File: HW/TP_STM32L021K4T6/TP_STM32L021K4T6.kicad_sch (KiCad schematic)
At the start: 16 parts, among them U1 STM32L021K4Tx, U2 BU33SD5WG-TR

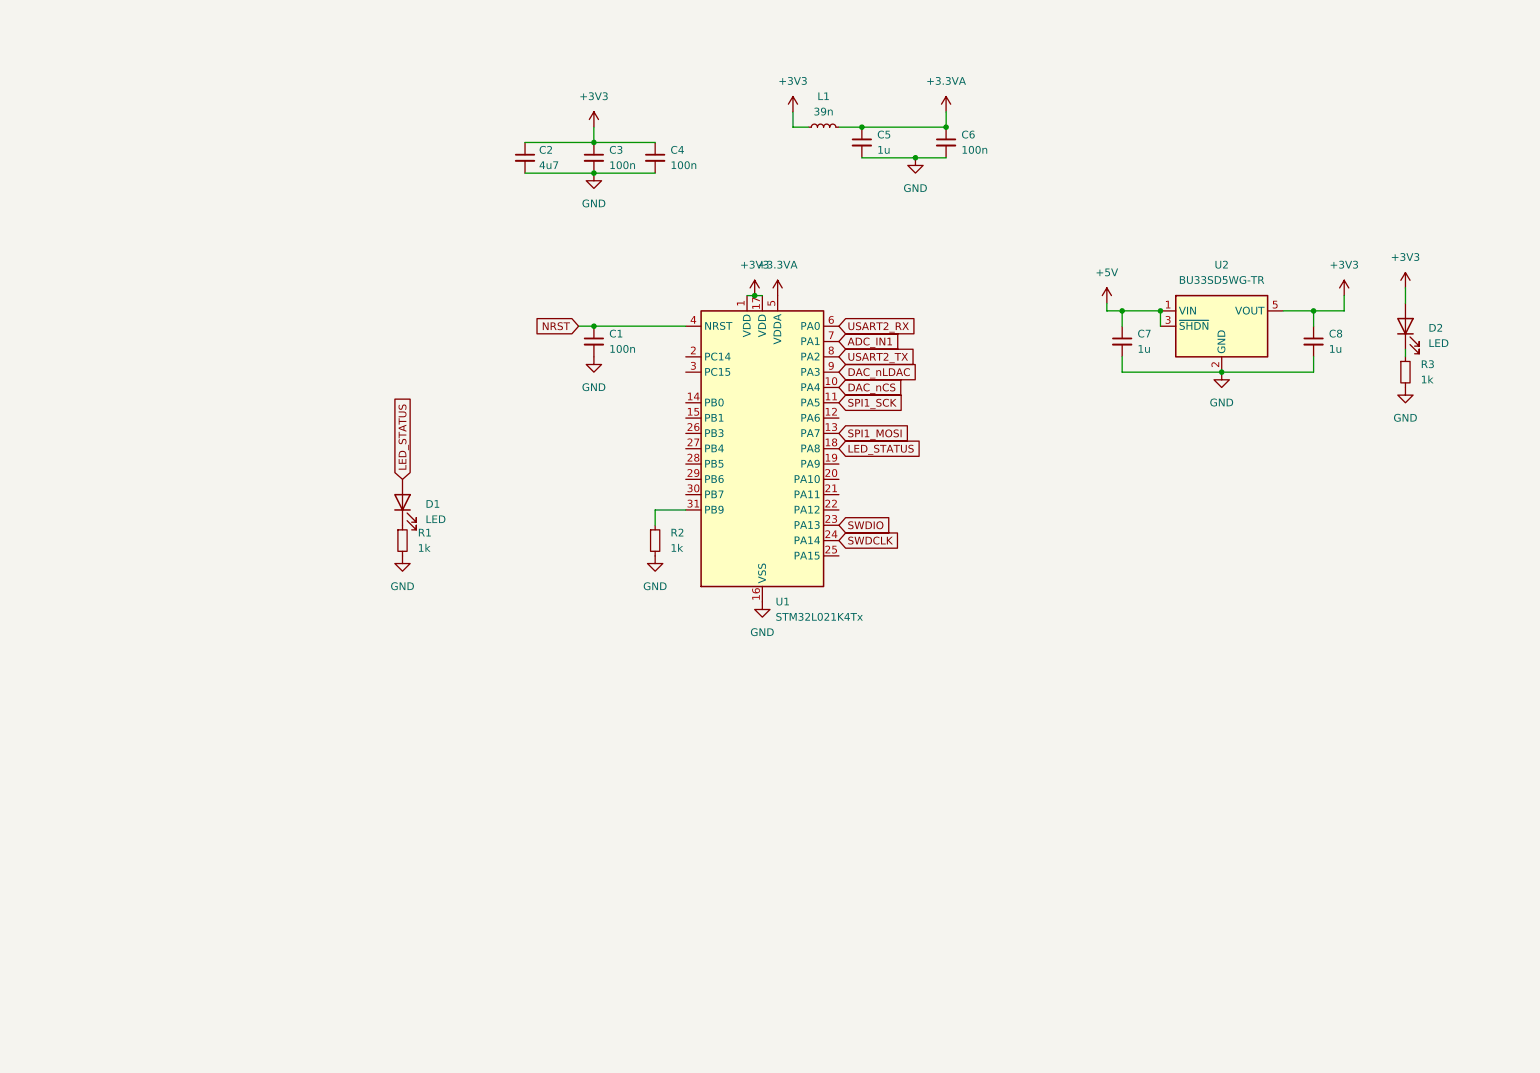
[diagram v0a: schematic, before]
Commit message: Save PCB
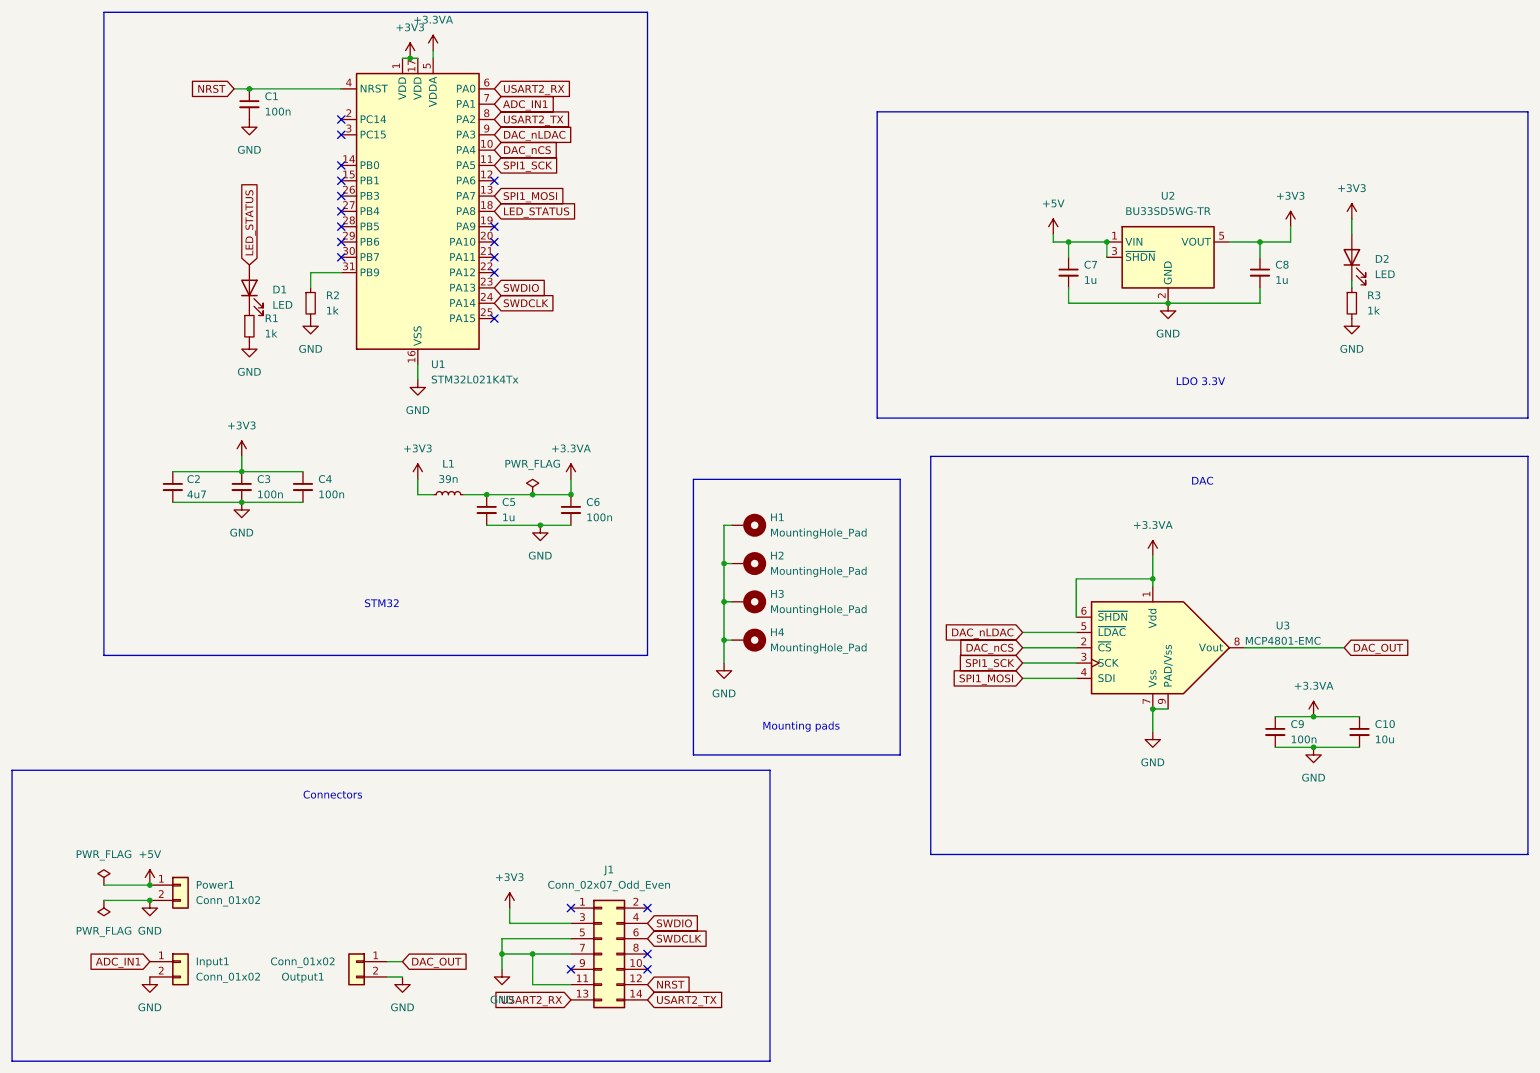
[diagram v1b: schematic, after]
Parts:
- added C10: 10u, Capacitor_SMD:C_0805_2012Metric, symbol Device:C_Small
- added C9: 100n, Capacitor_SMD:C_0805_2012Metric_Pad1.18x1.45mm_HandSolder, symbol Device:C_Small
- added H1, H2, H3, H4: MountingHole_Pad, MountingHole:MountingHole_3.2mm_M3_Pad, symbol Mechanical:MountingHole_Pad
- added Input1, Output1, Power1: Conn_01x02, Connector_JST:JST_XH_B2B-XH-AM_1x02_P2.50mm_Vertical, symbol Connector_Generic:Conn_01x02
- added J1: Conn_02x07_Odd_Even, Connector_PinHeader_1.27mm:PinHeader_2x07_P1.27mm_Vertical_SMD, symbol Connector_Generic:Conn_02x07_Odd_Even
- added U3: MCP4801-EMC, Package_DFN_QFN:DFN-8-1EP_3x2mm_P0.5mm_EP1.75x1.45mm, symbol Analog_DAC:MCP4801-EMC
- C1, C2, C3, C4, C6: footprint (none) -> Capacitor_SMD:C_0805_2012Metric_Pad1.18x1.45mm_HandSolder
- C5, C7, C8: footprint (none) -> Capacitor_SMD:C_0805_2012Metric
- D1, D2: footprint (none) -> LED_SMD:LED_0201_0603Metric_Pad0.64x0.40mm_HandSolder
- L1: footprint (none) -> Inductor_SMD:L_0805_2012Metric_Pad1.05x1.20mm_HandSolder
- R1, R2, R3: footprint (none) -> Resistor_SMD:R_0805_2012Metric_Pad1.20x1.40mm_HandSolder
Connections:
- net +3.3VA: now also C10.1, C9.1, U3.1 (Vdd), U3.6 (~{SHDN})
- net +3V3: now also J1.3 (Pin_3)
- net +5V: now also Power1.1 (Pin_1)
- net ADC_IN1: now also Input1.1 (Pin_1)
- net DAC_nCS: now also U3.2 (~{CS})
- net DAC_nLDAC: now also U3.5 (~{LDAC})
- net GND: now also C10.2, C9.2, H1.1, H2.1, H3.1, H4.1, Input1.2 (Pin_2), J1.11 (Pin_11), J1.5 (Pin_5), J1.7 (Pin_7), Output1.2 (Pin_2), Power1.2 (Pin_2), U3.7 (Vss), U3.9 (PAD/Vss)
- net NRST: now also J1.12 (Pin_12)
- net SPI1_MOSI: now also U3.4 (SDI)
- net SPI1_SCK: now also U3.3 (SCK)
- net SWDCLK: now also J1.6 (Pin_6)
- net SWDIO: now also J1.4 (Pin_4)
- net USART2_RX: now also J1.13 (Pin_13)
- net USART2_TX: now also J1.14 (Pin_14)
- new net DAC_OUT: Output1.1 (Pin_1), U3.8 (Vout)
- no-connect marks 0 -> 20
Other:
- note added: "Connectors"
- note added: "DAC"
- note added: "LDO 3.3V"
- note added: "Mounting pads"
- note added: "STM32"
- moved on the sheet: C1, C2, C3, C4, C5, C6, C7, C8, D1, D2, L1, R1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

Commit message: firware
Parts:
- D1, D2: footprint LED_SMD:LED_0201_0603Metric_Pad0.64x0.40mm_HandSolder -> LED_SMD:LED_0603_1608Metric_Pad1.05x0.95mm_HandSolder
- Input1, Output1, Power1: footprint Connector_JST:JST_XH_B2B-XH-AM_1x02_P2.50mm_Vertical -> Connector_JST:JST_XH_B2B-XH-A_1x02_P2.50mm_Vertical
- U3: footprint Package_DFN_QFN:DFN-8-1EP_3x2mm_P0.5mm_EP1.75x1.45mm -> Package_SO:SOIC-8_3.9x4.9mm_P1.27mm
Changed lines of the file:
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@@
       (effects (font (size 1.27 1.27)) (justify right))
     )
-    (property "Footprint" "LED_SMD:LED_0201_0603Metric_Pad0.64x0.40mm_HandSolder" (at 59.69 58.42 0)
+    (property "Footprint" "LED_SMD:LED_0603_1608Metric_Pad1.05x0.95mm_HandSolder" (at 59.69 58.42 0)
       (effects (font (size 1.27 1.27)) hide)
     )
@@
       (effects (font (size 1.27 1.27)) (justify right))
     )
-    (property "Footprint" "LED_SMD:LED_0201_0603Metric_Pad0.64x0.40mm_HandSolder" (at 242.57 53.34 0)
+    (property "Footprint" "LED_SMD:LED_0603_1608Metric_Pad1.05x0.95mm_HandSolder" (at 242.57 53.34 0)
       (effects (font (size 1.27 1.27)) hide)
     )
@@
       (effects (font (size 1.27 1.27)))
     )
-    (property "Footprint" "Connector_JST:JST_XH_B2B-XH-AM_1x02_P2.50mm_Vertical" (at 77.47 170.18 0)
+    (property "Footprint" "Connector_JST:JST_XH_B2B-XH-A_1x02_P2.50mm_Vertical" (at 77.47 170.18 0)
       (effects (font (size 1.27 1.27)) hide)
     )
@@
       (effects (font (size 1.27 1.27)) (justify left))
     )
-    (property "Footprint" "Connector_JST:JST_XH_B2B-XH-AM_1x02_P2.50mm_Vertical" (at 48.26 170.18 0)
+    (property "Footprint" "Connector_JST:JST_XH_B2B-XH-A_1x02_P2.50mm_Vertical" (at 48.26 170.18 0)
       (effects (font (size 1.27 1.27)) hide)
     )
@@
       (effects (font (size 1.27 1.27)) (justify left))
     )
-    (property "Footprint" "Connector_JST:JST_XH_B2B-XH-AM_1x02_P2.50mm_Vertical" (at 48.26 157.48 0)
+    (property "Footprint" "Connector_JST:JST_XH_B2B-XH-A_1x02_P2.50mm_Vertical" (at 48.26 157.48 0)
       (effects (font (size 1.27 1.27)) hide)
     )
@@
       (effects (font (size 1.27 1.27)))
     )
-    (property "Footprint" "Package_DFN_QFN:DFN-8-1EP_3x2mm_P0.5mm_EP1.75x1.45mm" (at 209.55 130.048 0)
-      (effects (font (size 1.27 1.27)) hide)
-    )
+    (property "Footprint" "Package_SO:SOIC-8_3.9x4.9mm_P1.27mm" (at 209.55 130.048 0)
+      (effects (font (size 1.27 1.27)) hide)
+    )
